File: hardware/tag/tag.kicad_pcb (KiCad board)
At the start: 2 copper layers, 50 x 52 mm, 118 parts, among them J1 USB_C_Receptacle_USB2.0_16P, J10 Conn_01x02, J2 BATTERY, J3 BLE_Conn, J4 SOURCE, J5 STM SWD, J6 I2C, J7 UART, J8 BLE SWD, J9 AUX, Q2 AO3400A, Q3 AO3401A, SW1 PWR, SW2 RESET, SW3 USER, U1 MAX17048G_T10, U2 USBLC6-2SC6, U3 ICM-45686, U4 TPS63070RNMR, U5 BQ24075RGT, U6 FSC-BT630, U7 STM32F411CEUx, U8 DWM1000, Y1 NX3215SA-32.768kHz(DNP), Y2 NX3225SA-24MHz

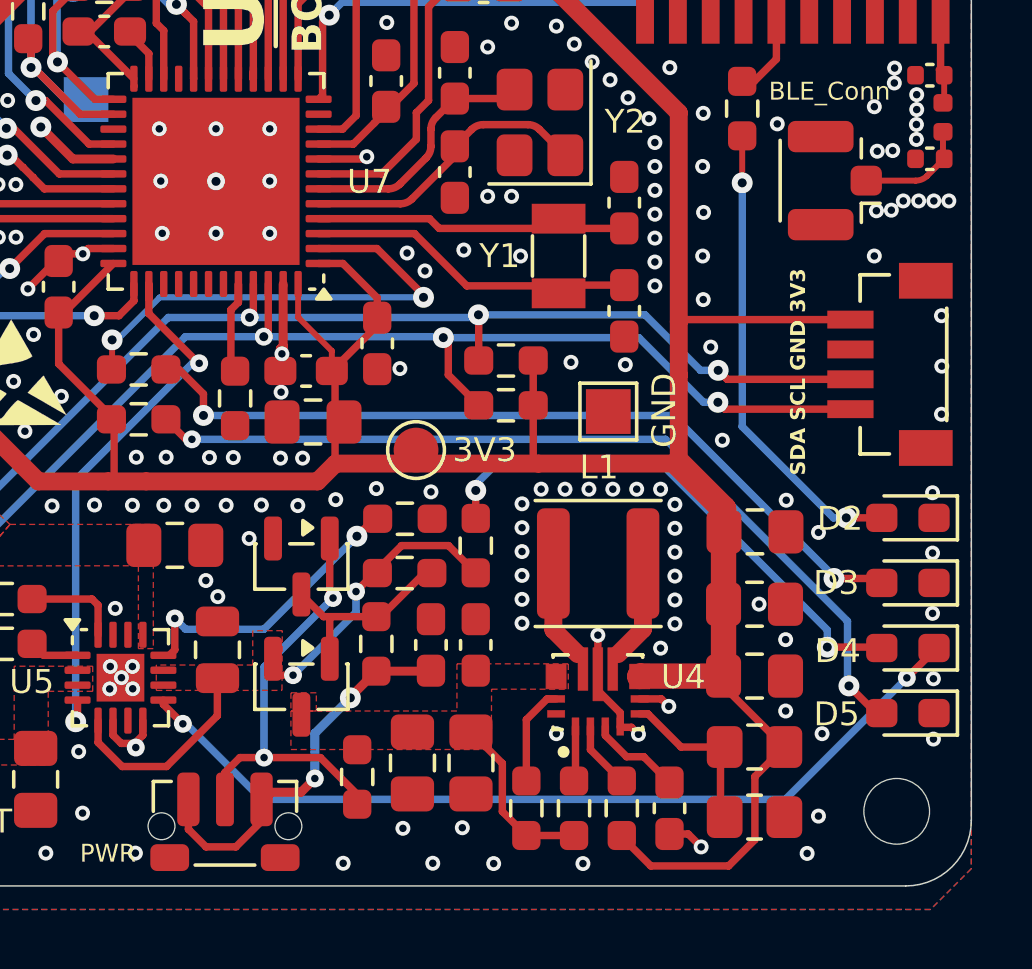
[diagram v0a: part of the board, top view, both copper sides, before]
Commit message: wip
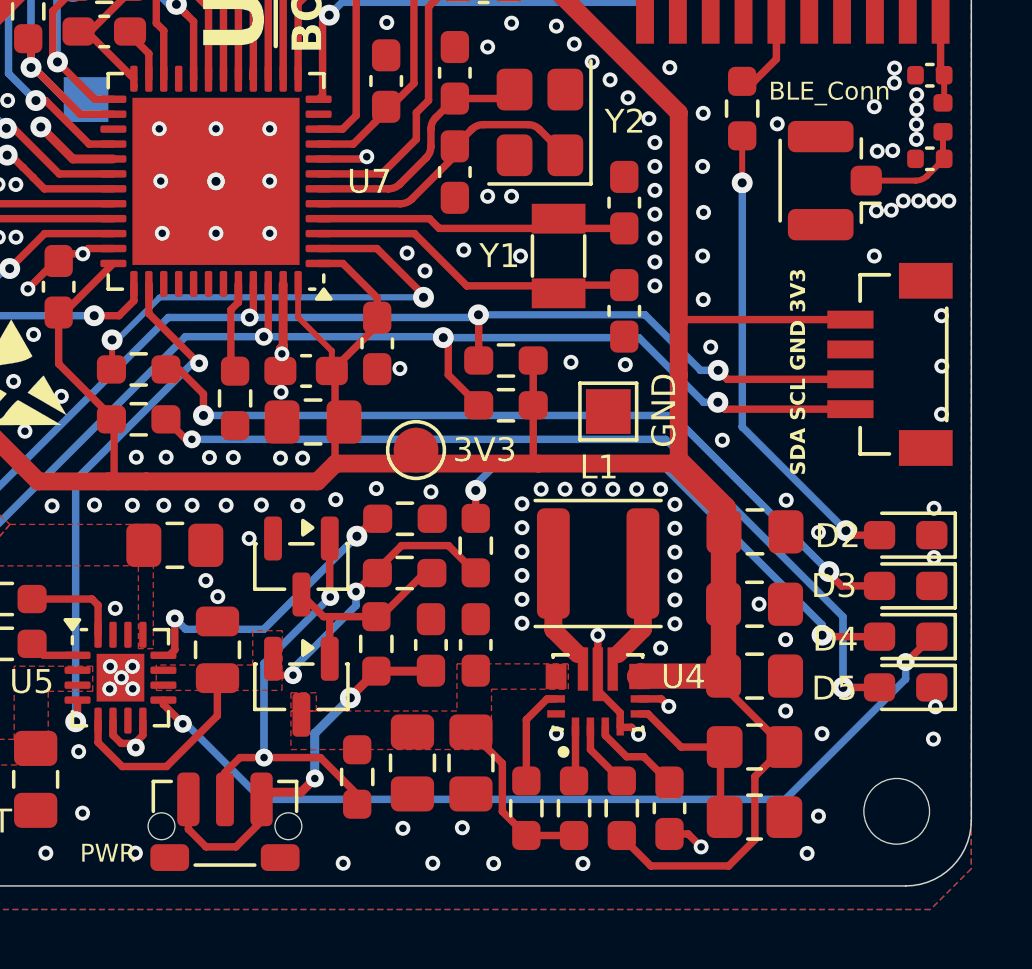
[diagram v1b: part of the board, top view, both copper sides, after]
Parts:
- moved D5 0.86 mm to (78.8, 95.5)
- moved D2 0.58 mm to (78.8, 90.3)
- moved D4 0.39 mm to (78.8, 93.8)
- moved D3 0.12 mm to (78.8, 92.0)
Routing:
- net Net-(D3-A): track 27.6 -> 28.3 mm
- net GND: vias 396 -> 395
